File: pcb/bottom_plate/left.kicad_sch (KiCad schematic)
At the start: 14 parts

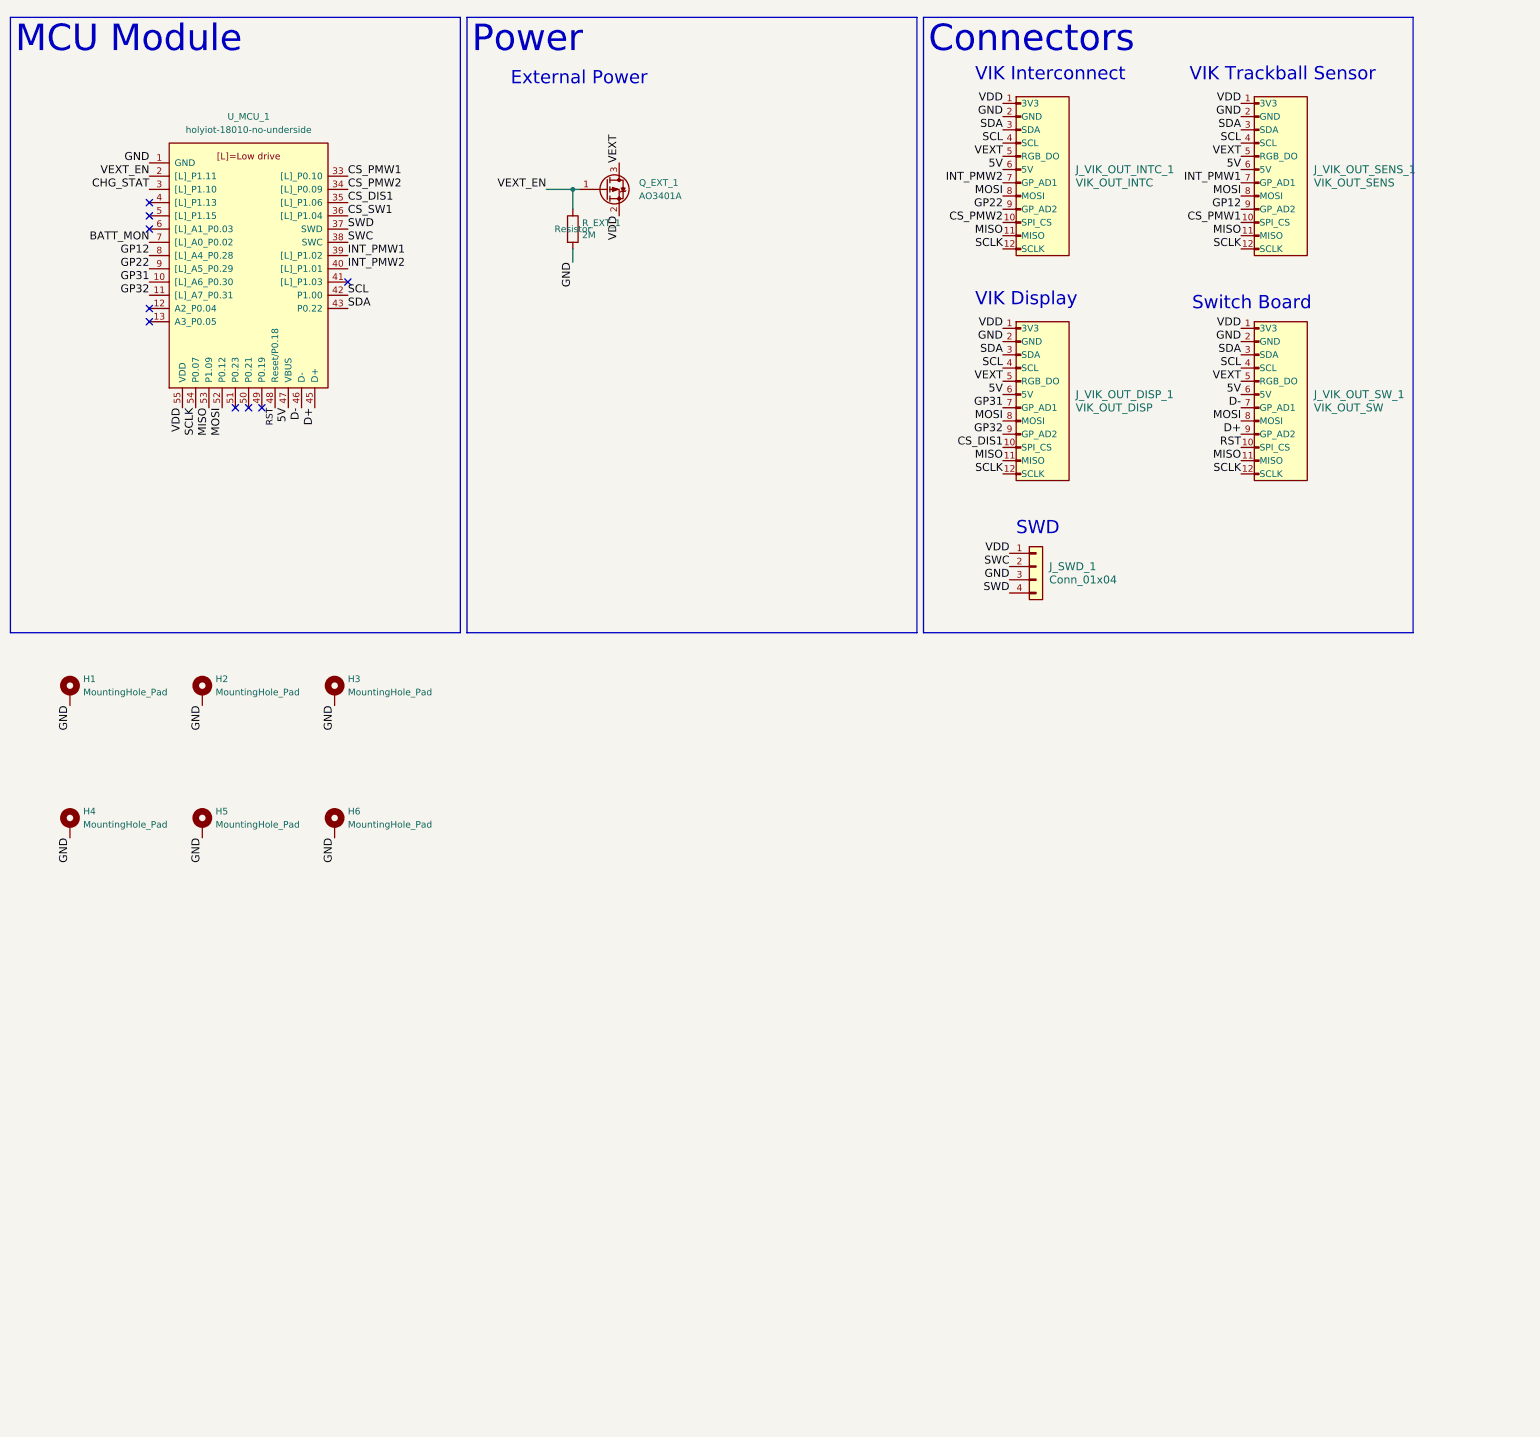
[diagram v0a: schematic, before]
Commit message: Start redoing bottom plate.
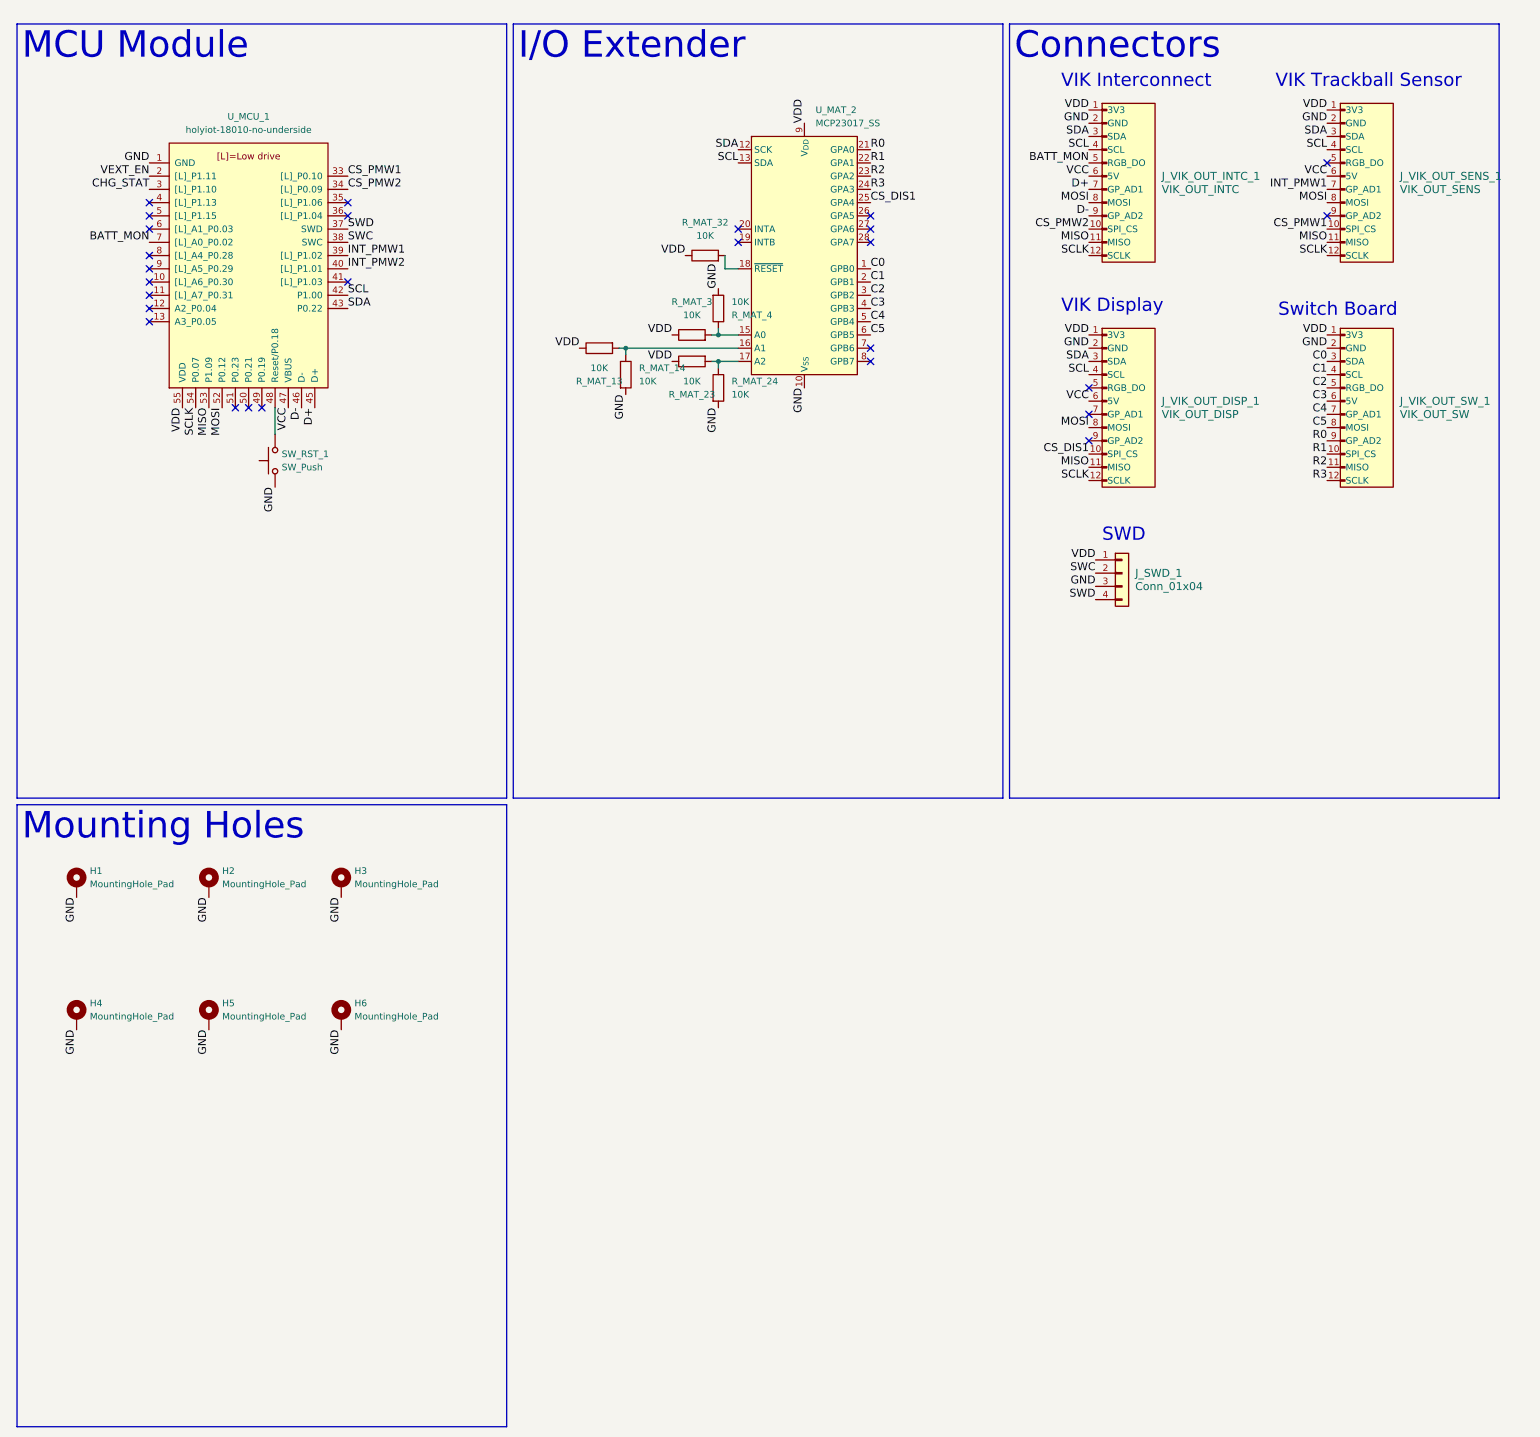
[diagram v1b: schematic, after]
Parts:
- removed Q_EXT_1: AO3401A, Package_TO_SOT_SMD:SOT-23, symbol Transistor_FET:AO3401A
- removed R_EXT_1: 2M, Resistor_SMD:R_0603_1608Metric, symbol Device:R
- added R_MAT_13, R_MAT_14, R_MAT_23, R_MAT_24, R_MAT_3, R_MAT_32, R_MAT_4: 10K, Resistor_SMD:R_0201_0603Metric_Pad0.64x0.40mm_HandSolder, symbol Device:R
- added SW_RST_1: SW_Push, Button_Switch_SMD:SW_Push_1P1T_NO_E-Switch_TL3301NxxxxxG, symbol Switch:SW_Push
- added U_MAT_2: MCP23017_SS, Package_SO:SSOP-28_5.3x10.2mm_P0.65mm, symbol Interface_Expansion:MCP23017x-x-SS
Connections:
- net BATT_MON: now also J_VIK_OUT_INTC_1.5 (RGB_DO)
- net CS_DIS1: now also U_MAT_2.25 (GPA4); no longer U_MCU_1.35 ([L]_P1.06)
- net D+: now also J_VIK_OUT_INTC_1.7 (GP_AD1); no longer J_VIK_OUT_SW_1.9 (GP_AD2)
- net D-: now also J_VIK_OUT_INTC_1.9 (GP_AD2); no longer J_VIK_OUT_SW_1.7 (GP_AD1)
- net GND: now also R_MAT_14.2, R_MAT_24.2, R_MAT_4.2, SW_RST_1.1, U_MAT_2.10 (V_{SS})
- net INT_PMW2: no longer J_VIK_OUT_INTC_1.7 (GP_AD1)
- net MISO: no longer J_VIK_OUT_SW_1.11 (MISO)
- net MOSI: no longer J_VIK_OUT_SW_1.8 (MOSI)
- net SCL: now also U_MAT_2.13 (SDA); no longer J_VIK_OUT_SW_1.4 (SCL)
- net SCLK: no longer J_VIK_OUT_SW_1.12 (SCLK)
- net SDA: now also U_MAT_2.12 (SCK); no longer J_VIK_OUT_SW_1.3 (SDA)
- net VDD: now also R_MAT_13.1, R_MAT_23.1, R_MAT_3.1, R_MAT_32.1, U_MAT_2.9 (V_{DD})
- net 5V renamed VCC
- net VCC: no longer J_VIK_OUT_SW_1.6 (5V)
- net CS_SW1: no longer names the net of U_MCU_1.36 ([L]_P1.04)
- net GP12: no longer names the net of J_VIK_OUT_SENS_1.9 (GP_AD2)
- net GP12: no longer U_MCU_1.8 ([L]_A4_P0.28)
- net GP22: no longer names the net of U_MCU_1.9 ([L]_A5_P0.29)
- net GP22: no longer J_VIK_OUT_INTC_1.9 (GP_AD2)
- net GP31: no longer names the net of J_VIK_OUT_DISP_1.7 (GP_AD1)
- net GP31: no longer U_MCU_1.10 ([L]_A6_P0.30)
- net GP32: no longer names the net of J_VIK_OUT_DISP_1.9 (GP_AD2)
- net GP32: no longer U_MCU_1.11 ([L]_A7_P0.31)
- net RST: no longer names the net of U_MCU_1.48 (Reset/P0.18)
- net RST: now also SW_RST_1.2; no longer J_VIK_OUT_SW_1.10 (SPI_CS)
- removed net VEXT: J_VIK_OUT_DISP_1.5 (RGB_DO), J_VIK_OUT_INTC_1.5 (RGB_DO), J_VIK_OUT_SENS_1.5 (RGB_DO), J_VIK_OUT_SW_1.5 (RGB_DO)
- new net: R_MAT_3.2, R_MAT_4.1, U_MAT_2.15 (A0)
- new net: R_MAT_23.2, R_MAT_24.1, U_MAT_2.17 (A2)
- new net: R_MAT_13.2, R_MAT_14.1, U_MAT_2.16 (A1)
- new net: R_MAT_32.2, U_MAT_2.18 (~{RESET})
- new net C0: J_VIK_OUT_SW_1.3 (SDA), U_MAT_2.1 (GPB0)
- new net C1: J_VIK_OUT_SW_1.4 (SCL), U_MAT_2.2 (GPB1)
- new net C2: J_VIK_OUT_SW_1.5 (RGB_DO), U_MAT_2.3 (GPB2)
- new net C3: J_VIK_OUT_SW_1.6 (5V), U_MAT_2.4 (GPB3)
- new net C4: J_VIK_OUT_SW_1.7 (GP_AD1), U_MAT_2.5 (GPB4)
- new net C5: J_VIK_OUT_SW_1.8 (MOSI), U_MAT_2.6 (GPB5)
- new net R0: J_VIK_OUT_SW_1.9 (GP_AD2), U_MAT_2.21 (GPA0)
- new net R1: J_VIK_OUT_SW_1.10 (SPI_CS), U_MAT_2.22 (GPA1)
- new net R2: J_VIK_OUT_SW_1.11 (MISO), U_MAT_2.23 (GPA2)
- new net R3: J_VIK_OUT_SW_1.12 (SCLK), U_MAT_2.24 (GPA3)
- no-connect marks 9 -> 27
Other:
- note removed: "External Power"
- moved on the sheet: H1, H2, H3, H4, H5, H6, J_SWD_1, J_VIK_OUT_DISP_1, J_VIK_OUT_INTC_1, J_VIK_OUT_SENS_1, J_VIK_OUT_SW_1
